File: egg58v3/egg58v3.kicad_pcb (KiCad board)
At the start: 2 copper layers, 141.1 x 127.1 mm, 37 parts, among them J1 AudioJack4, SW11 SW_PUSH_LED, SW12 SW_PUSH_LED, SW13 SW_PUSH_LED, SW14 SW_PUSH_LED, SW15 SW_PUSH_LED, SW16 SW_PUSH_LED, SW21 SW_PUSH_LED, SW22 SW_PUSH_LED, SW23 SW_PUSH_LED, SW24 SW_PUSH_LED, SW25 SW_PUSH_LED, SW26 SW_PUSH_LED, SW31 SW_PUSH_LED, SW32 SW_PUSH_LED, SW33 SW_PUSH_LED, SW34 SW_PUSH_LED, SW35 SW_PUSH_LED, SW36 SW_PUSH_LED, SW41 SW_PUSH_LED, SW42 SW_PUSH_LED, SW43 SW_PUSH_LED, SW44 SW_PUSH_LED, SW45 SW_PUSH_LED, SW46 SW_PUSH_LED, SW52 SW_PUSH_LED, SW53 SW_PUSH_LED, SW54 SW_PUSH_LED, SW55 SW_PUSH_LED, SW56 SW_PUSH_LED, U1 Elite-C

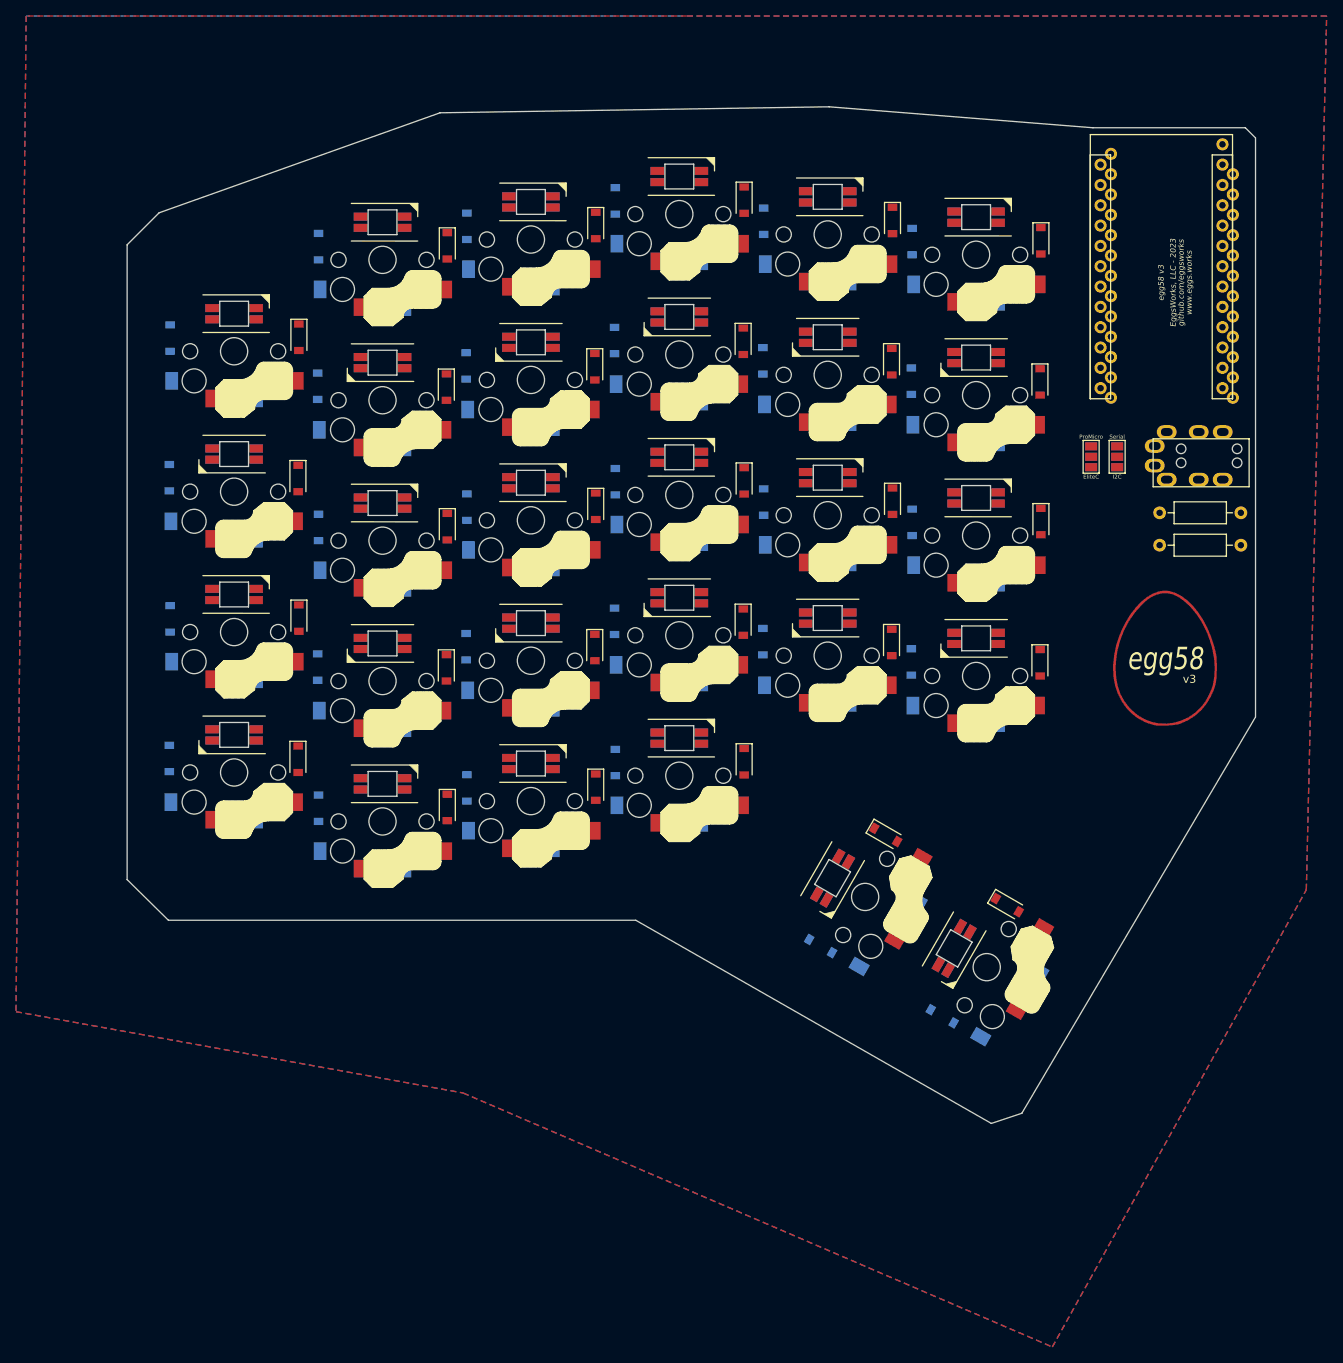
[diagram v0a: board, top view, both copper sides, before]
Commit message: Initial layout for v3
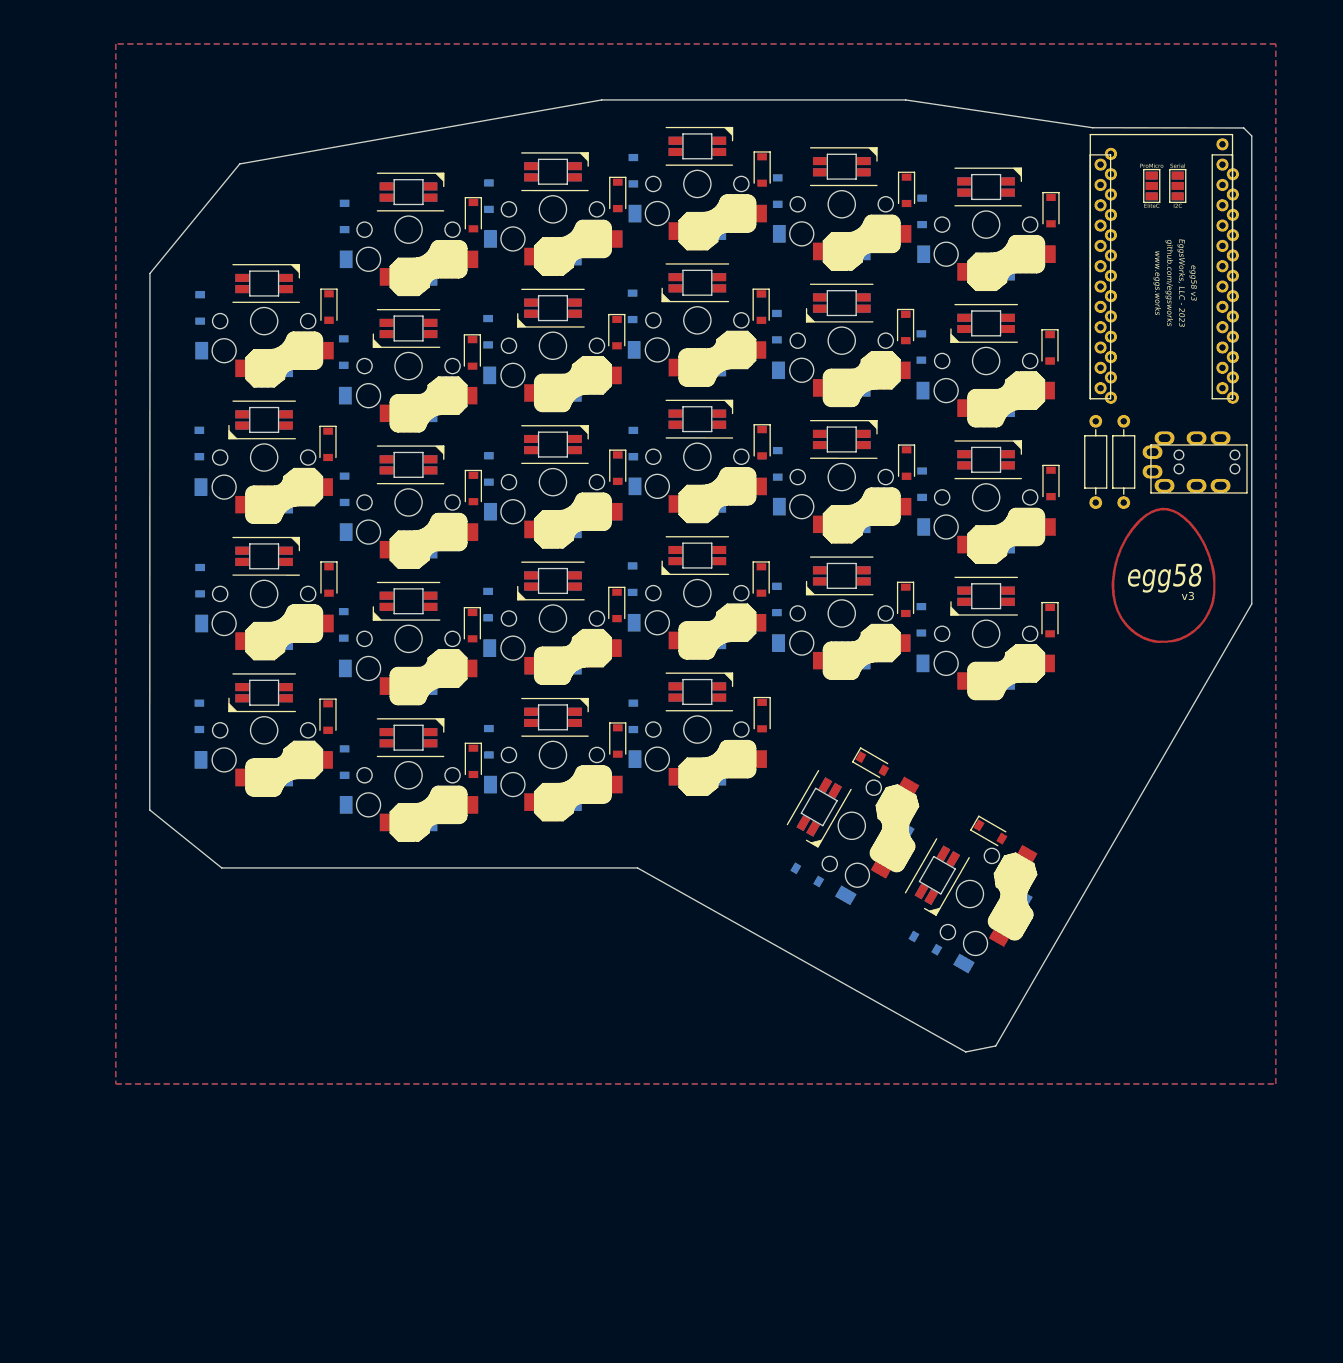
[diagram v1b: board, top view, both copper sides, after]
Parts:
- SW55, SW56: footprint egg58v2:Choc_Hotswap_SK6812MiniE -> egg58v2:Choc_Hotswap_SK6812MiniE_Thumb
- moved JP1 34.7 mm to (164.5, 47.8)
- moved JP2 34.7 mm to (167.8, 47.8)
- moved #LOGO1 10.4 mm to (166.0, 96.5)
- moved R2 9.59 mm to (157.5, 87.3), turned to 90 degrees
- moved SW56 9.38 mm to (141.8, 136.3)
- moved SW55 9.05 mm to (127.0, 127.7)
- moved SW52 6.63 mm to (71.6, 121.4)
- moved SW41 6.47 mm to (53.5, 115.8)
- moved SW53 6.39 mm to (89.7, 118.9)
- moved SW54 6.20 mm to (107.7, 115.7)
- moved SW42 6.19 mm to (71.6, 104.4)
- moved SW31 6.07 mm to (53.5, 98.7)
- moved SW43 5.95 mm to (89.7, 101.8)
- moved SW32 5.78 mm to (71.6, 87.3)
- moved SW44 5.73 mm to (107.7, 98.7)
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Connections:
- SW11 pad 10: (no net) -> GND
- SW11 pad 11: (no net) -> Net-(SW11-Pad11)
- SW11 pad 12: (no net) -> Col1
- SW11 pad 13: (no net) -> Net-(SW11-Pad13)
- SW11 pad 14: (no net) -> Row1
- SW11 pad 8: (no net) -> VCC
- SW11 pad 9: (no net) -> Net-(SW11-Pad9)
- SW12 pad 10: (no net) -> GND
- SW12 pad 11: (no net) -> Net-(SW12-Pad11)
- SW12 pad 12: (no net) -> Col2
- SW12 pad 13: (no net) -> Net-(SW12-Pad13)
- SW12 pad 14: (no net) -> Row1
- SW12 pad 8: (no net) -> VCC
- SW12 pad 9: (no net) -> Net-(SW11-Pad11)
- SW13 pad 10: (no net) -> GND
- SW13 pad 11: (no net) -> Net-(SW13-Pad11)
- SW13 pad 12: (no net) -> Col3
- SW13 pad 13: (no net) -> Net-(SW13-Pad13)
- SW13 pad 14: (no net) -> Row1
- SW13 pad 8: (no net) -> VCC
- SW13 pad 9: (no net) -> Net-(SW12-Pad11)
- SW14 pad 10: (no net) -> GND
- SW14 pad 11: (no net) -> Net-(SW14-Pad11)
- SW14 pad 12: (no net) -> Col4
- SW14 pad 13: (no net) -> Net-(SW14-Pad13)
- SW14 pad 14: (no net) -> Row1
- SW14 pad 8: (no net) -> VCC
- SW14 pad 9: (no net) -> Net-(SW13-Pad11)
- SW15 pad 10: (no net) -> GND
- SW15 pad 11: (no net) -> Net-(SW15-Pad11)
- SW15 pad 12: (no net) -> Col5
- SW15 pad 13: (no net) -> Net-(SW15-Pad13)
- SW15 pad 14: (no net) -> Row1
- SW15 pad 8: (no net) -> VCC
- SW15 pad 9: (no net) -> Net-(SW14-Pad11)
- SW16 pad 10: (no net) -> GND
- SW16 pad 11: (no net) -> RGB
- SW16 pad 12: (no net) -> Col6
- SW16 pad 13: (no net) -> Net-(SW16-Pad13)
- SW16 pad 14: (no net) -> Row1
- SW16 pad 8: (no net) -> VCC
- SW16 pad 9: (no net) -> Net-(SW15-Pad11)
- SW21 pad 10: (no net) -> GND
- SW21 pad 11: (no net) -> Net-(SW11-Pad9)
- SW21 pad 12: (no net) -> Col1
- SW21 pad 13: (no net) -> Net-(SW21-Pad13)
- SW21 pad 14: (no net) -> Row2
- SW21 pad 8: (no net) -> VCC
- SW21 pad 9: (no net) -> Net-(SW21-Pad9)
- SW22 pad 10: (no net) -> GND
- SW22 pad 11: (no net) -> Net-(SW21-Pad9)
- SW22 pad 12: (no net) -> Col2
- SW22 pad 13: (no net) -> Net-(SW22-Pad13)
- SW22 pad 14: (no net) -> Row2
- SW22 pad 8: (no net) -> VCC
- SW22 pad 9: (no net) -> Net-(SW22-Pad9)
- SW23 pad 10: (no net) -> GND
- SW23 pad 11: (no net) -> Net-(SW22-Pad9)
- SW23 pad 12: (no net) -> Col3
- SW23 pad 13: (no net) -> Net-(SW23-Pad13)
- SW23 pad 14: (no net) -> Row2
- SW23 pad 8: (no net) -> VCC
- SW23 pad 9: (no net) -> Net-(SW23-Pad9)
- SW24 pad 10: (no net) -> GND
- SW24 pad 11: (no net) -> Net-(SW23-Pad9)
- SW24 pad 12: (no net) -> Col4
- SW24 pad 13: (no net) -> Net-(SW24-Pad13)
- SW24 pad 14: (no net) -> Row2
- SW24 pad 8: (no net) -> VCC
- SW24 pad 9: (no net) -> Net-(SW24-Pad9)
- SW25 pad 10: (no net) -> GND
- SW25 pad 11: (no net) -> Net-(SW24-Pad9)
- SW25 pad 12: (no net) -> Col5
- SW25 pad 13: (no net) -> Net-(SW25-Pad13)
- SW25 pad 14: (no net) -> Row2
- SW25 pad 8: (no net) -> VCC
- SW25 pad 9: (no net) -> Net-(SW25-Pad9)
- SW26 pad 10: (no net) -> GND
- SW26 pad 11: (no net) -> Net-(SW25-Pad9)
- SW26 pad 12: (no net) -> Col6
- SW26 pad 13: (no net) -> Net-(SW26-Pad13)
- SW26 pad 14: (no net) -> Row2
- SW26 pad 8: (no net) -> VCC
- SW26 pad 9: (no net) -> Net-(SW26-Pad9)
- SW31 pad 10: (no net) -> GND
- SW31 pad 11: (no net) -> Net-(SW31-Pad11)
- SW31 pad 12: (no net) -> Col1
- SW31 pad 13: (no net) -> Net-(SW31-Pad13)
- SW31 pad 14: (no net) -> Row3
- SW31 pad 8: (no net) -> VCC
- SW31 pad 9: (no net) -> Net-(SW31-Pad9)
- SW32 pad 10: (no net) -> GND
- SW32 pad 11: (no net) -> Net-(SW32-Pad11)
- SW32 pad 12: (no net) -> Col2
- SW32 pad 13: (no net) -> Net-(SW32-Pad13)
- SW32 pad 14: (no net) -> Row3
- SW32 pad 8: (no net) -> VCC
- SW32 pad 9: (no net) -> Net-(SW31-Pad11)
- SW33 pad 10: (no net) -> GND
- SW33 pad 11: (no net) -> Net-(SW33-Pad11)
- SW33 pad 12: (no net) -> Col3
- SW33 pad 13: (no net) -> Net-(SW33-Pad13)
- SW33 pad 14: (no net) -> Row3
- SW33 pad 8: (no net) -> VCC
- SW33 pad 9: (no net) -> Net-(SW32-Pad11)
- SW34 pad 10: (no net) -> GND
- SW34 pad 11: (no net) -> Net-(SW34-Pad11)
- SW34 pad 12: (no net) -> Col4
- SW34 pad 13: (no net) -> Net-(SW34-Pad13)
- SW34 pad 14: (no net) -> Row3
- SW34 pad 8: (no net) -> VCC
- SW34 pad 9: (no net) -> Net-(SW33-Pad11)
- SW35 pad 10: (no net) -> GND
- SW35 pad 11: (no net) -> Net-(SW35-Pad11)
- SW35 pad 12: (no net) -> Col5
- SW35 pad 13: (no net) -> Net-(SW35-Pad13)
- SW35 pad 14: (no net) -> Row3
- SW35 pad 8: (no net) -> VCC
- SW35 pad 9: (no net) -> Net-(SW34-Pad11)
- SW36 pad 10: (no net) -> GND
- SW36 pad 11: (no net) -> Net-(SW26-Pad9)
- SW36 pad 12: (no net) -> Col6
- SW36 pad 13: (no net) -> Net-(SW36-Pad13)
- SW36 pad 14: (no net) -> Row3
- SW36 pad 8: (no net) -> VCC
- SW36 pad 9: (no net) -> Net-(SW35-Pad11)
- SW41 pad 10: (no net) -> GND
- SW41 pad 11: (no net) -> Net-(SW31-Pad9)
- SW41 pad 12: (no net) -> Col1
- SW41 pad 13: (no net) -> Net-(SW41-Pad13)
- SW41 pad 14: (no net) -> Row4
- SW41 pad 8: (no net) -> VCC
- SW41 pad 9: (no net) -> Net-(SW41-Pad9)
- SW42 pad 10: (no net) -> GND
- SW42 pad 11: (no net) -> Net-(SW41-Pad9)
- SW42 pad 12: (no net) -> Col2
- SW42 pad 13: (no net) -> Net-(SW42-Pad13)
- SW42 pad 14: (no net) -> Row4
- SW42 pad 8: (no net) -> VCC
- SW42 pad 9: (no net) -> Net-(SW42-Pad9)
- SW43 pad 10: (no net) -> GND
- SW43 pad 11: (no net) -> Net-(SW42-Pad9)
- SW43 pad 12: (no net) -> Col3
- SW43 pad 13: (no net) -> Net-(SW43-Pad13)
- SW43 pad 14: (no net) -> Row4
- SW43 pad 8: (no net) -> VCC
- SW43 pad 9: (no net) -> Net-(SW43-Pad9)
- SW44 pad 10: (no net) -> GND
- SW44 pad 11: (no net) -> Net-(SW43-Pad9)
- SW44 pad 12: (no net) -> Col4
- SW44 pad 13: (no net) -> Net-(SW44-Pad13)
- SW44 pad 14: (no net) -> Row4
- SW44 pad 8: (no net) -> VCC
- SW44 pad 9: (no net) -> Net-(SW44-Pad9)
- SW45 pad 10: (no net) -> GND
- SW45 pad 11: (no net) -> Net-(SW44-Pad9)
- SW45 pad 12: (no net) -> Col5
- SW45 pad 13: (no net) -> Net-(SW45-Pad13)
- SW45 pad 14: (no net) -> Row4
- SW45 pad 8: (no net) -> VCC
- SW45 pad 9: (no net) -> Net-(SW45-Pad9)
- SW46 pad 10: (no net) -> GND
- SW46 pad 11: (no net) -> Net-(SW45-Pad9)
- SW46 pad 12: (no net) -> Col6
- SW46 pad 13: (no net) -> Net-(SW46-Pad13)
- SW46 pad 14: (no net) -> Row4
- SW46 pad 8: (no net) -> VCC
- SW46 pad 9: (no net) -> Net-(SW46-Pad9)
- SW52 pad 10: (no net) -> GND
- SW52 pad 11: (no net) -> Net-(SW52-Pad11)
- SW52 pad 12: (no net) -> Col2
- SW52 pad 13: (no net) -> Net-(SW52-Pad13)
- SW52 pad 14: (no net) -> Row5
- SW52 pad 8: (no net) -> VCC
- SW52 pad 9: (no net) -> unconnected-(SW52-Pad9)
- SW53 pad 10: (no net) -> GND
- SW53 pad 11: (no net) -> Net-(SW53-Pad11)
- SW53 pad 12: (no net) -> Col3
- SW53 pad 13: (no net) -> Net-(SW53-Pad13)
- SW53 pad 14: (no net) -> Row5
- SW53 pad 8: (no net) -> VCC
- SW53 pad 9: (no net) -> Net-(SW52-Pad11)
- SW54 pad 10: (no net) -> GND
- SW54 pad 11: (no net) -> Net-(SW54-Pad11)
- SW54 pad 12: (no net) -> Col4
- SW54 pad 13: (no net) -> Net-(SW54-Pad13)
- SW54 pad 14: (no net) -> Row5
- SW54 pad 8: (no net) -> VCC
- SW54 pad 9: (no net) -> Net-(SW53-Pad11)
- SW55 pad 10: (no net) -> GND
- SW55 pad 11: (no net) -> Net-(SW55-Pad11)
- SW55 pad 12: (no net) -> Col5
- SW55 pad 13: (no net) -> Net-(SW55-Pad13)
- SW55 pad 14: (no net) -> Row5
- SW55 pad 8: (no net) -> VCC
- SW55 pad 9: (no net) -> Net-(SW54-Pad11)
- SW56 pad 10: (no net) -> GND
- SW56 pad 11: (no net) -> Net-(SW46-Pad9)
- SW56 pad 12: (no net) -> Col6
- SW56 pad 13: (no net) -> Net-(SW56-Pad13)
- SW56 pad 14: (no net) -> Row5
- SW56 pad 8: (no net) -> VCC
- SW56 pad 9: (no net) -> Net-(SW55-Pad11)
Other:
- board size 141.1 x 127.1 mm -> 137.8 x 119 mm
